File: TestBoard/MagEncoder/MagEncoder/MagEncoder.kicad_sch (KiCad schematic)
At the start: 5 parts, among them J1 Conn_01x07, U1 AS5050A

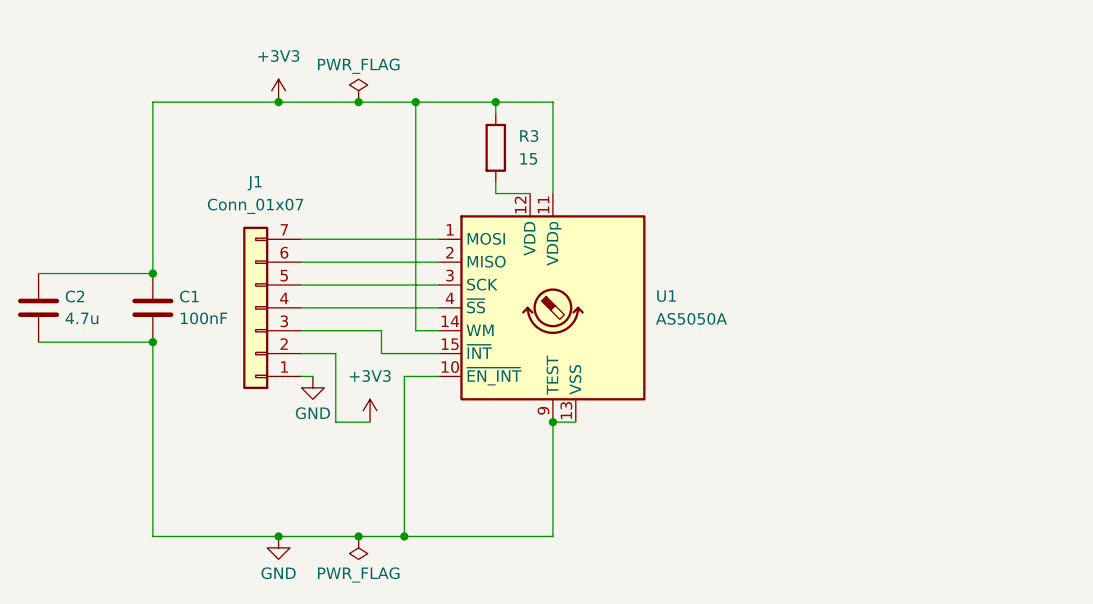
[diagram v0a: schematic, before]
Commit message: Mag Encoder Done
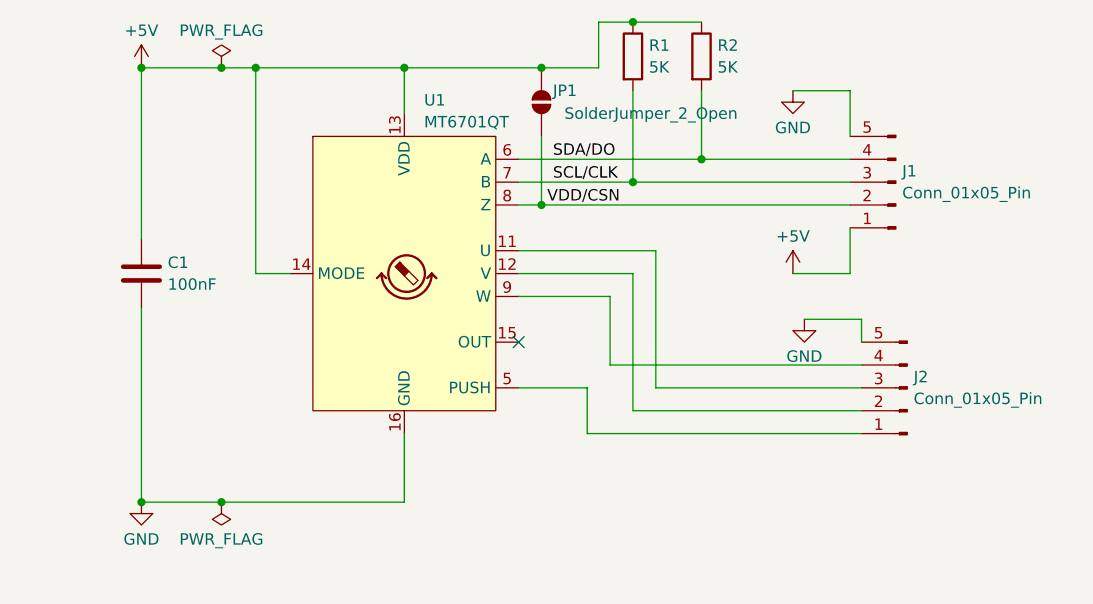
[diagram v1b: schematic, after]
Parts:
- removed C2: 4.7u, Capacitor_SMD:C_0402_1005Metric, symbol Device:C
- removed J1: Conn_01x07, symbol Connector_Generic:Conn_01x07
- removed R3: 15, Resistor_SMD:R_0402_1005Metric, symbol Device:R
- removed U1: AS5050A, Package_DFN_QFN:QFN-16-1EP_4x4mm_P0.65mm_EP2.7x2.7mm_PullBack, symbol Sensor_Magnetic:AS5050A
- added J1, J2: Conn_01x05_Pin, Connector_JST:JST_GH_SM05B-GHS-TB_1x05-1MP_P1.25mm_Horizontal, symbol Connector:Conn_01x05_Pin
- added JP1: SolderJumper_2_Open, Jumper:SolderJumper-2_P1.3mm_Bridged_RoundedPad1.0x1.5mm, symbol Jumper:SolderJumper_2_Open
- added R1, R2: 5K, Resistor_SMD:R_0603_1608Metric_Pad0.98x0.95mm_HandSolder, symbol Device:R
- added U1: MT6701QT, Package_DFN_QFN:QFN-16-1EP_3x3mm_P0.5mm_EP1.7x1.7mm, symbol Sensor_Magnetic:MT6701QT
- C1: footprint Capacitor_SMD:C_0402_1005Metric -> Capacitor_SMD:C_0805_2012Metric_Pad1.18x1.45mm_HandSolder
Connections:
- net GND: now also J1.5 (Pin_5), J2.5 (Pin_5), U1.16 (GND), U1.17 (GND)
- net +3V3 renamed +5V
- net +5V: now also J1.1 (Pin_1), JP1.2 (B), R1.1, R2.1, U1.13 (VDD), U1.14 (MODE)
- new net: J2.1 (Pin_1), U1.5 (PUSH)
- new net: J2.2 (Pin_2), U1.12 (V)
- new net: J2.3 (Pin_3), U1.11 (U)
- new net: J2.4 (Pin_4), U1.9 (W)
- new net SCL/CLK: J1.3 (Pin_3), R1.2, U1.7 (B)
- new net SDA/DO: J1.4 (Pin_4), R2.2, U1.6 (A)
- new net VDD/CSN: J1.2 (Pin_2), JP1.1 (A), U1.8 (Z)
- no-connect marks 0 -> 1
